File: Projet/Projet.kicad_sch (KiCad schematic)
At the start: 4 parts

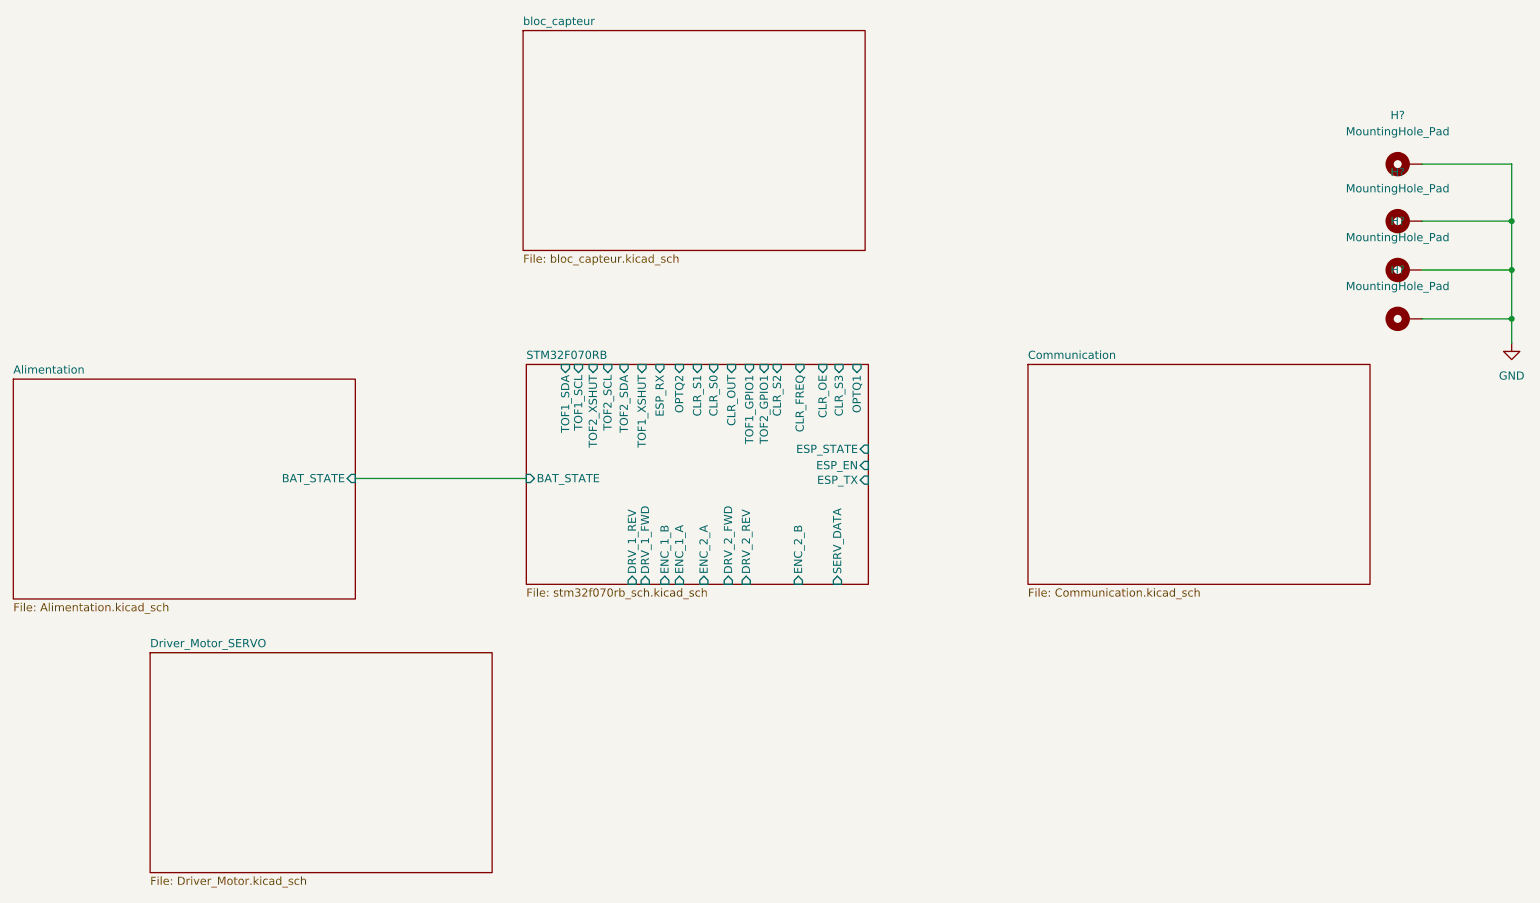
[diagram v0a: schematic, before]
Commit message: board_schematic
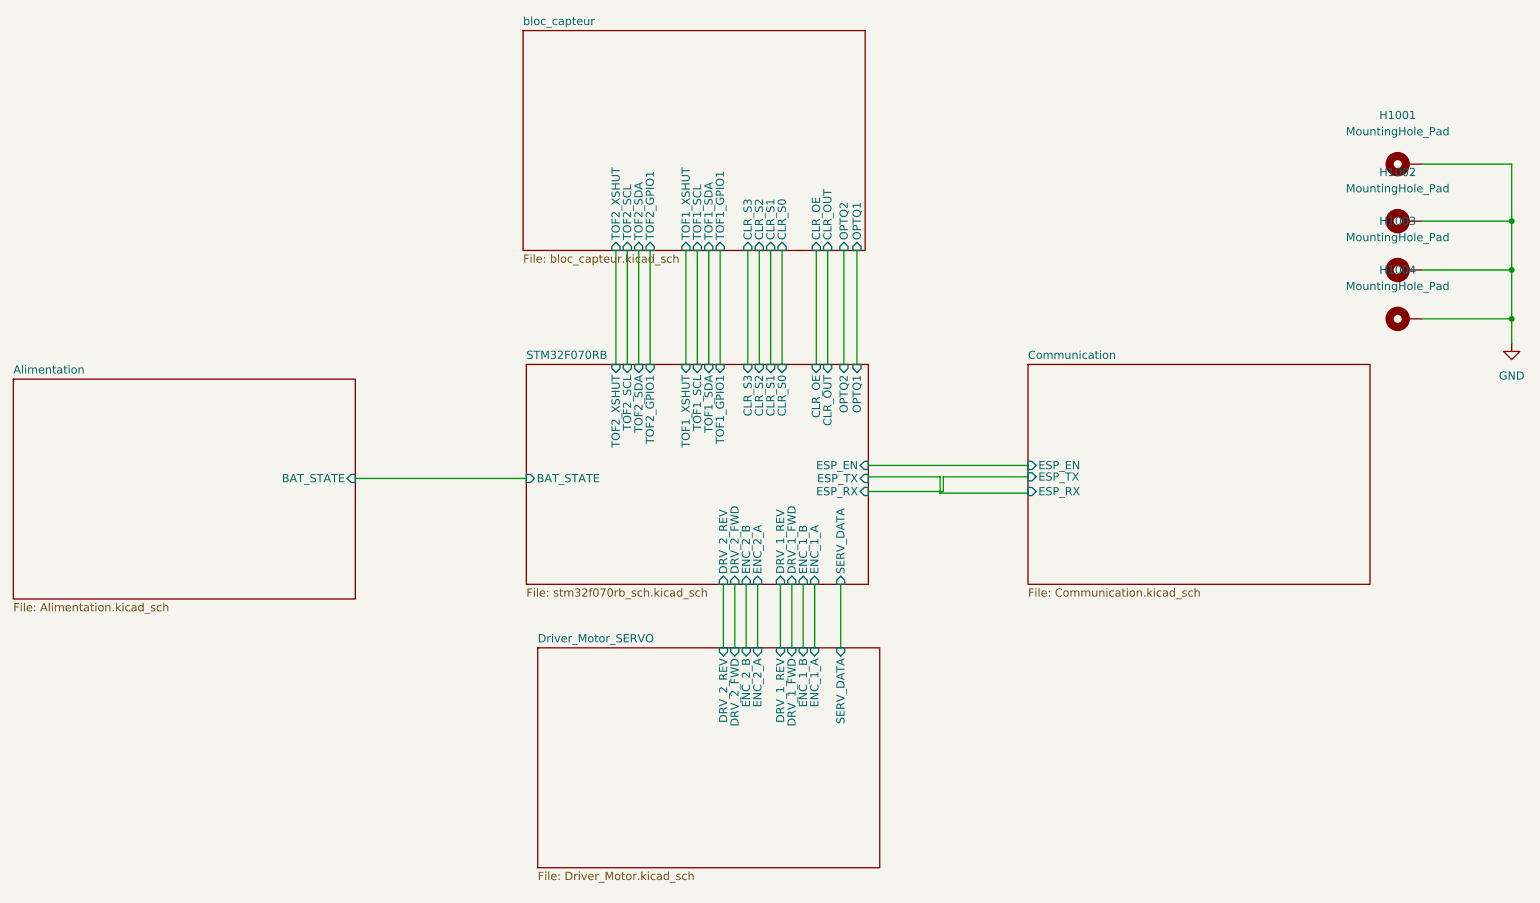
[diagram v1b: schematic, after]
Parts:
- H1001, H1002, H1003, H1004: renamed from H?; footprint (none) -> MountingHole:MountingHole_3.2mm_M3_Pad_Via
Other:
- sheet Communication ports: added ESP_EN, ESP_RX, ESP_TX; removed none
- sheet Driver_Motor_SERVO ports: added DRV_1_FWD, DRV_1_REV, DRV_2_FWD, DRV_2_REV, ENC_1_A, ENC_1_B, ENC_2_A, ENC_2_B, SERV_DATA; removed none
- sheet STM32F070RB ports: added none; removed CLR_FREQ, ESP_STATE
- sheet bloc_capteur ports: added CLR_OE, CLR_OUT, CLR_S0, CLR_S1, CLR_S2, CLR_S3, OPTQ1, OPTQ2, TOF1_GPIO1, TOF1_SCL, TOF1_SDA, TOF1_XSHUT, TOF2_GPIO1, TOF2_SCL, TOF2_SDA, TOF2_XSHUT; removed none
